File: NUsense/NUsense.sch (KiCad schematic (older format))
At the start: 3 parts

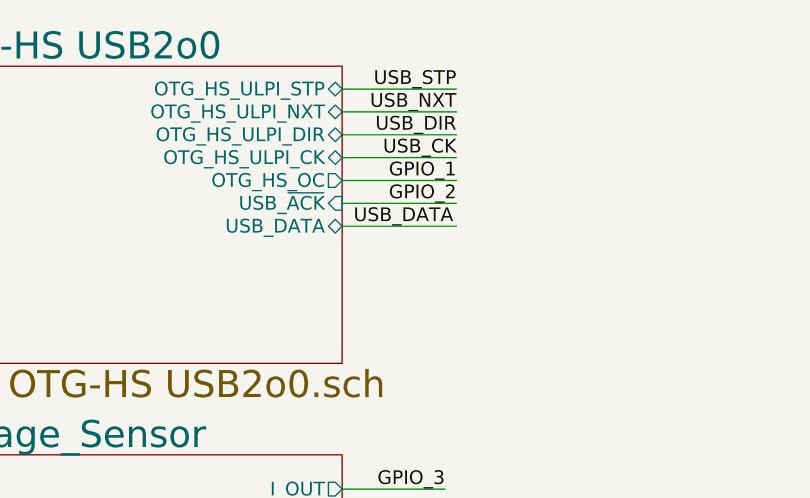
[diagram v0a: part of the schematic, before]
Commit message: Further Cleaning
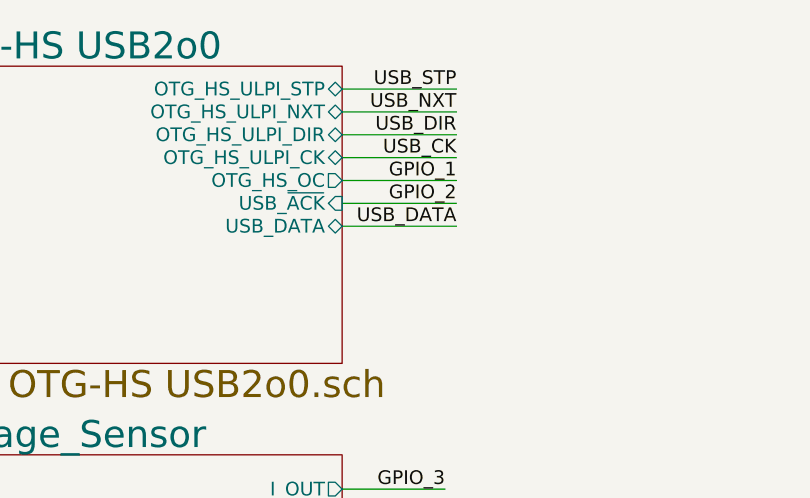
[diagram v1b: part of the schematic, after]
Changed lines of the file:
@@
 Wire Wire Line
 	4200 1850 4700 1850
-Text Label 4250 1850 0    60   ~ 0
+Text Label 4700 1850 2    60   ~ 0
 USB_DATA
 Wire Wire Line
